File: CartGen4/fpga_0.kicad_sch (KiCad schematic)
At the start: 13 parts, among them U9 LFXP2-8E-5MN132C

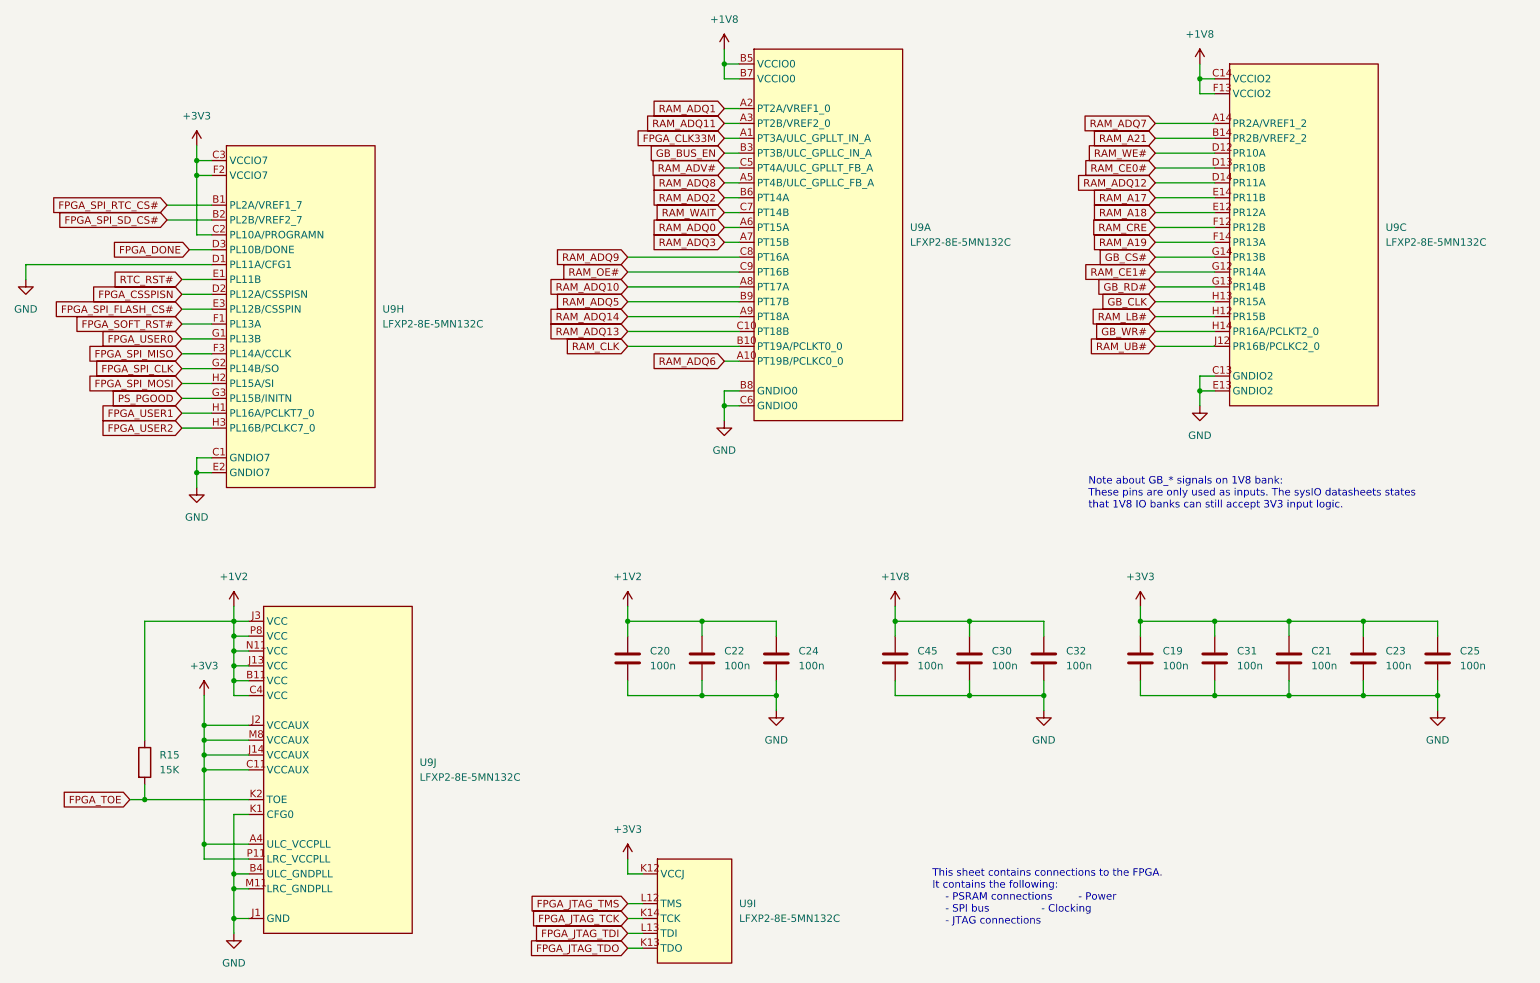
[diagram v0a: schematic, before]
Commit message: Minor adjustments
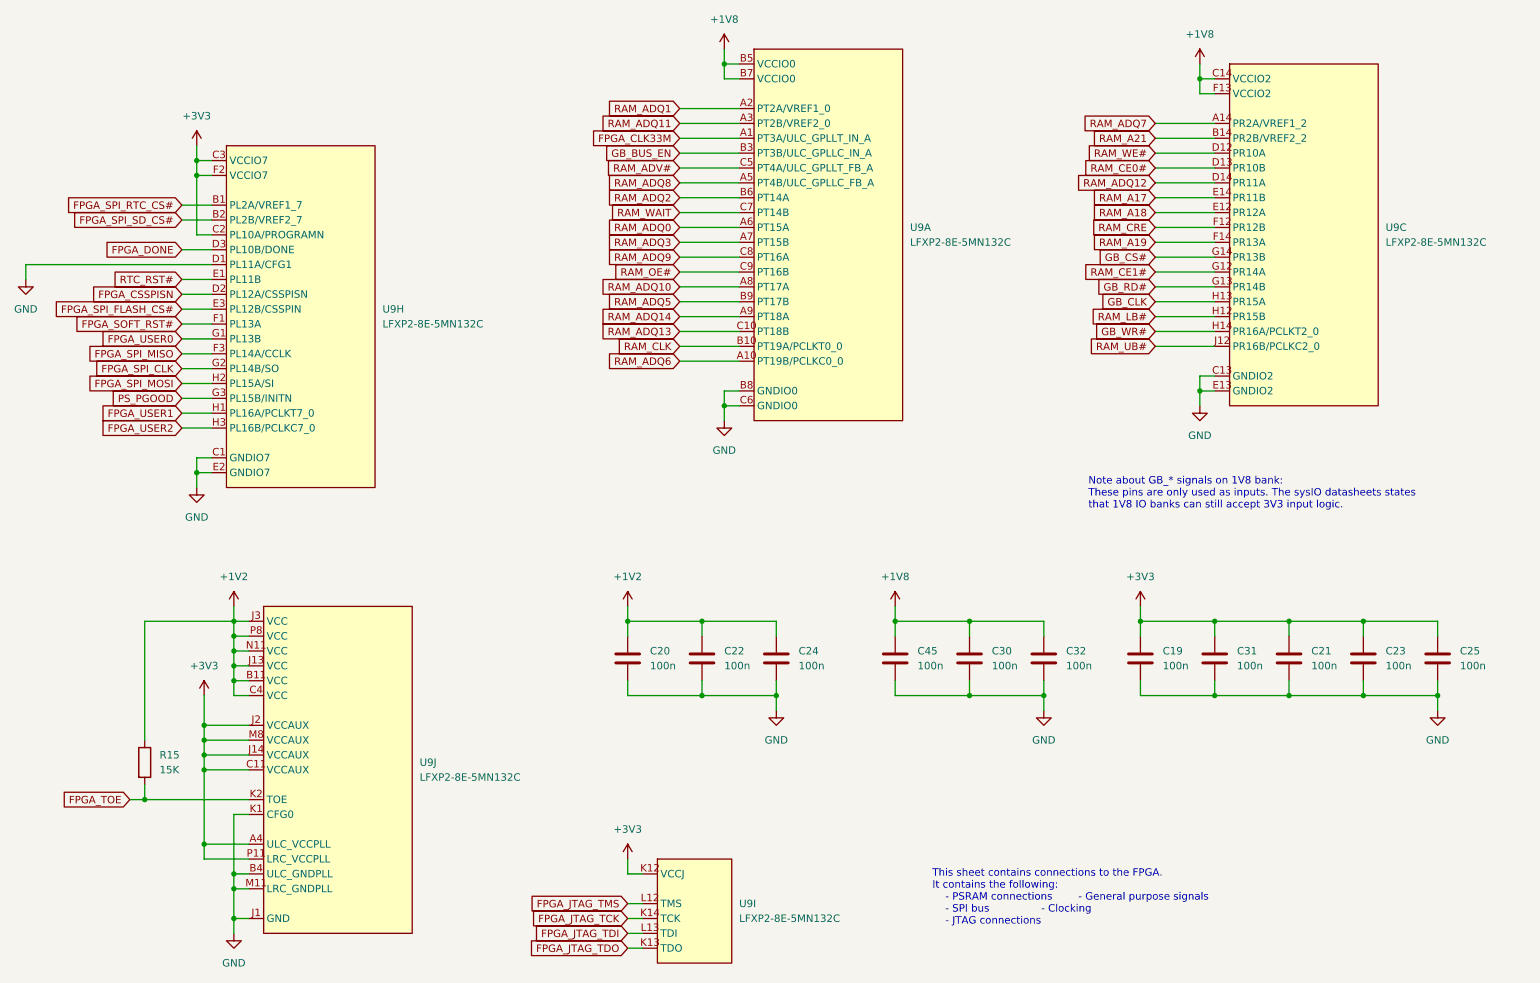
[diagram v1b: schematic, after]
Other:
- note added: "This sheet contains connections to the FPGA. It contains the following: - PSRAM connections - General purpose signals - SPI bus - Clocking - JTAG connections"
- note removed: "This sheet contains connections to the FPGA. It contains the following: - PSRAM connections - Power - SPI bus - Clocking - JTAG connections"
